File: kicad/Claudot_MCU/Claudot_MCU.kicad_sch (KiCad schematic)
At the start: 34 parts, among them J1 TYPE-C-31-M-12, J2 Conn_01x12, U1 RP2040, U2 W25Q16JVUXIQ, U3 AP2112K-3.3, Y1 12MHz

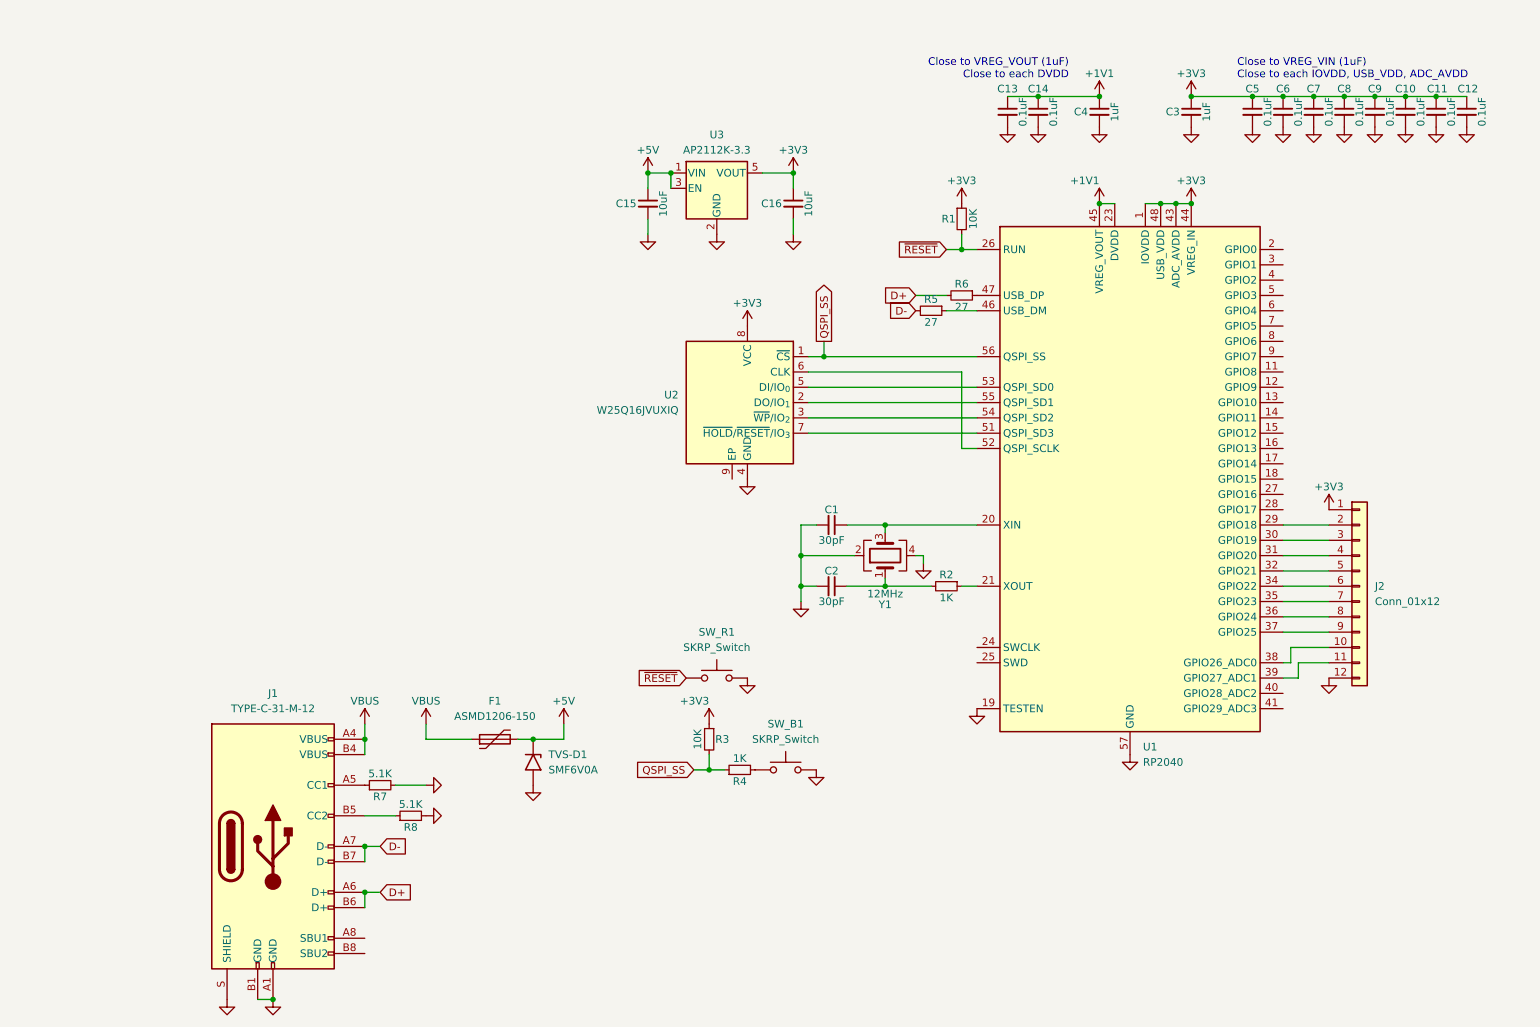
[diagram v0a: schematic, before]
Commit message: Update schematic and pcb
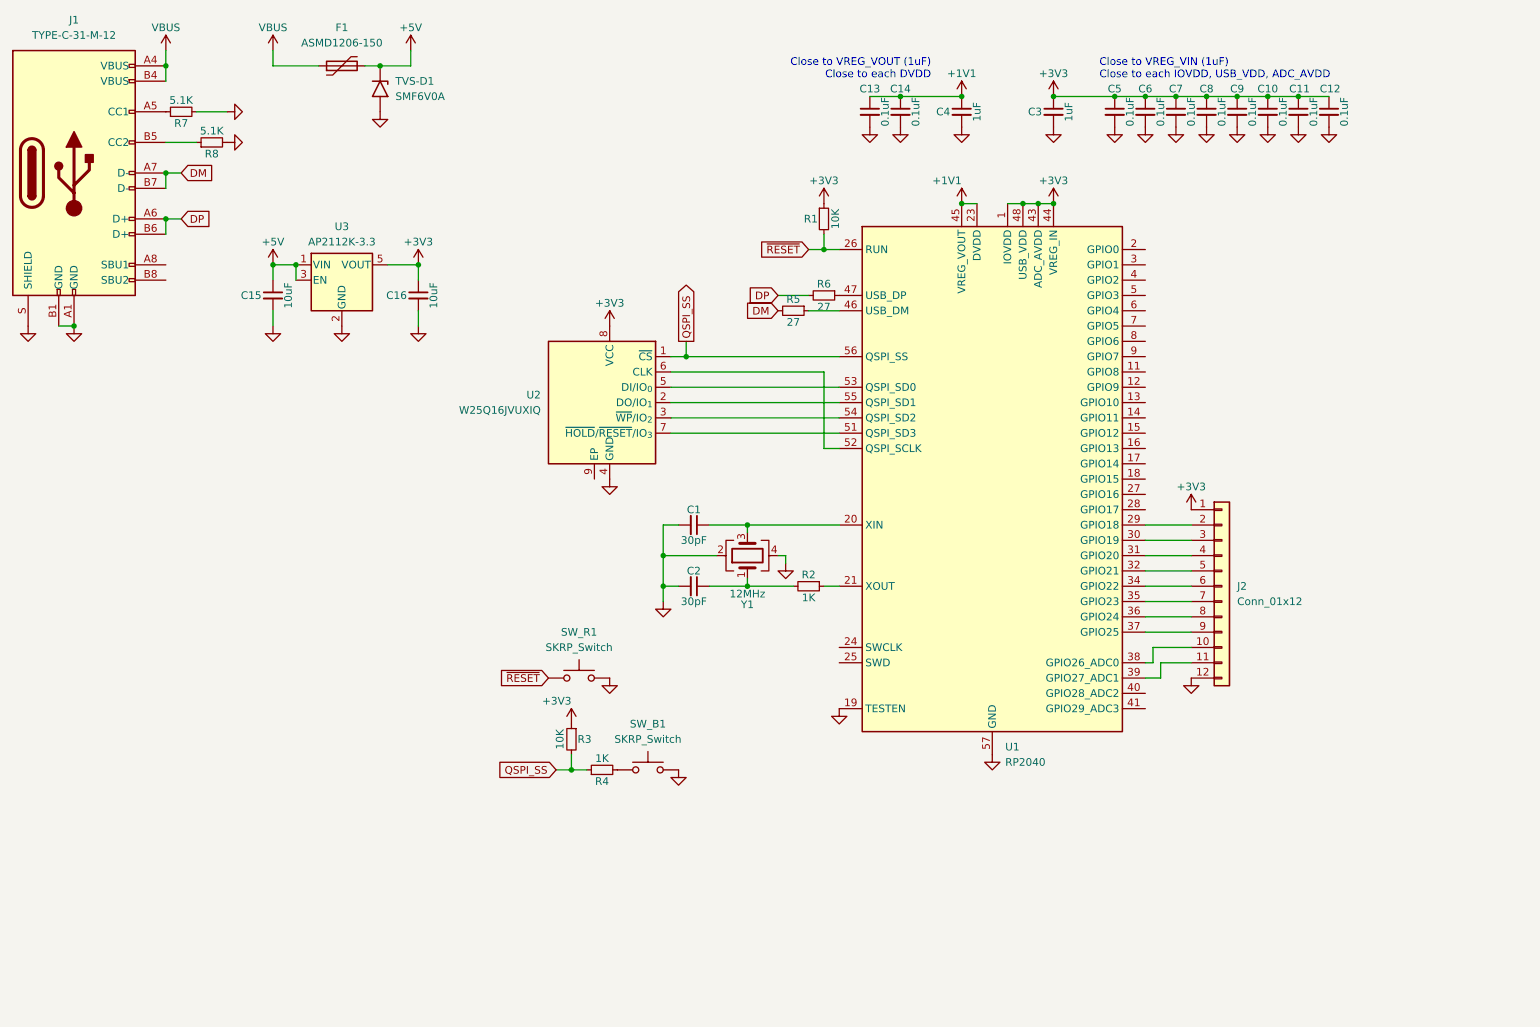
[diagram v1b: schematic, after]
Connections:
- net D+ renamed DP
- net D- renamed DM
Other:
- moved on the sheet: C1, C10, C11, C12, C13, C14, C15, C16, C2, C3, C4, C5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
